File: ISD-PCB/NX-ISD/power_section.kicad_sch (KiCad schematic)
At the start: 31 parts, among them P1 S2B-PH-SM4-TB, Q2 AO3401A, Q3 BC847W, U11 HYCW275-USBC24-050B, U13 RT9193-18GB, U15 USBLC6-2P6, U2 NCP167BMX330TBG, U8 BQ25170DSGR, U9 RT9193-28GB

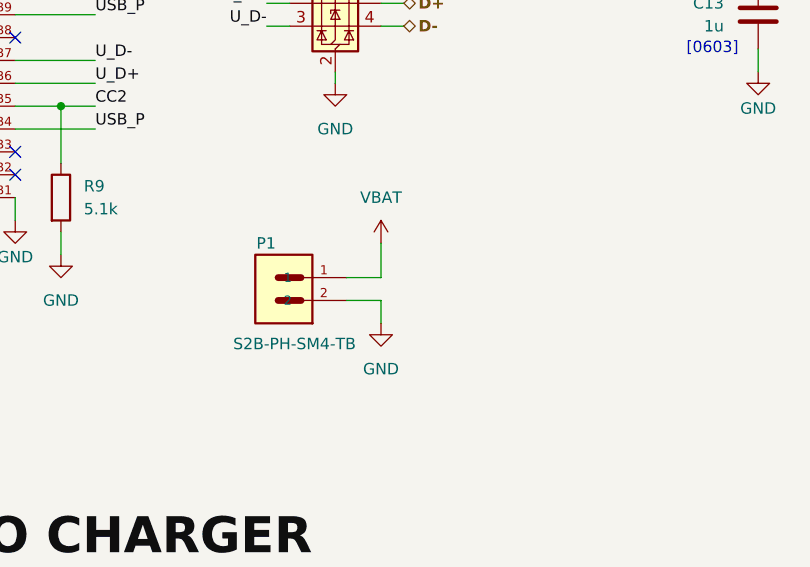
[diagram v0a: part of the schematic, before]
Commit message: v1p1 rework in progress
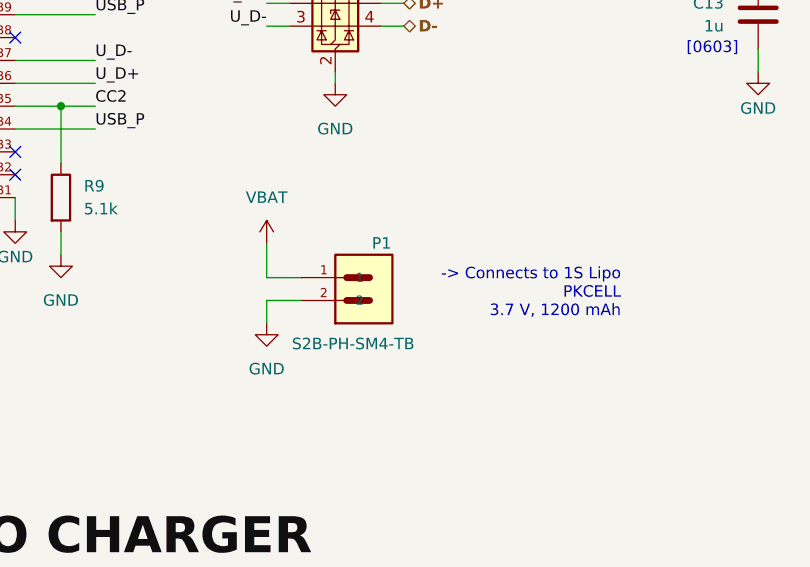
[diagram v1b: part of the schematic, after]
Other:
- note added: "-> Connects to 1S Lipo PKCELL 3.7 V, 1200 mAh"
- moved on the sheet: P1
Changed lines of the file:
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@@
 		)
 	)
+	(text "-> Connects to 1S Lipo\nPKCELL\n3.7 V, 1200 mAh"
+		(exclude_from_sim no)
+		(at 139.7 79.248 0)
+		(effects
+			(font
+				(size 1.27 1.27)
+			)
+			(justify right)
+		)
+	)
 	(text "[0603]"
 		(exclude_from_sim no)
@@
 	(wire
 		(pts
-			(xy 109.22 77.47) (xy 113.03 77.47)
+			(xy 104.14 77.47) (xy 100.33 77.47)
 		)
 		(stroke
@@
 	(wire
 		(pts
-			(xy 109.22 80.01) (xy 113.03 80.01)
+			(xy 104.14 80.01) (xy 100.33 80.01)
 		)
 		(stroke
@@
 	(wire
 		(pts
-			(xy 113.03 73.66) (xy 113.03 77.47)
+			(xy 100.33 73.66) (xy 100.33 77.47)
 		)
 		(stroke
@@
 	(wire
 		(pts
-			(xy 113.03 82.55) (xy 113.03 80.01)
+			(xy 100.33 82.55) (xy 100.33 80.01)
 		)
 		(stroke
@@
 	(symbol
 		(lib_id "power:GND")
-		(at 113.03 82.55 0)
+		(at 100.33 82.55 0)
+		(mirror y)
 		(unit 1)
 		(body_style 1)
@@
 		(fields_autoplaced yes)
 		(property "Reference" "#PWR013"
-			(at 113.03 88.9 0)
+			(at 100.33 88.9 0)
 			(hide yes)
 			(show_name no)
@@
 		)
 		(property "Value" "GND"
-			(at 113.03 87.63 0)
+			(at 100.33 87.63 0)
 			(show_name no)
 			(do_not_autoplace no)
@@
 		)
 		(property "Footprint" ""
-			(at 113.03 82.55 0)
+			(at 100.33 82.55 0)
 			(hide yes)
 			(show_name no)
@@
 		)
 		(property "Datasheet" ""
-			(at 113.03 82.55 0)
+			(at 100.33 82.55 0)
 			(hide yes)
 			(show_name no)
@@
 		)
 		(property "Description" "Power symbol creates a global label with name \"GND\" , ground"
-			(at 113.03 82.55 0)
+			(at 100.33 82.55 0)
 			(hide yes)
 			(show_name no)
@@
 	(symbol
 		(lib_id "S2B-PH-SM4-TB:S2B-PH-SM4-TB")
-		(at 104.14 78.74 0)
-		(mirror y)
+		(at 109.22 78.74 0)
 		(unit 1)
 		(body_style 1)
@@
 		(dnp no)
 		(property "Reference" "P1"
-			(at 101.346 73.66 0)
+			(at 112.014 73.66 0)
 			(show_name no)
 			(do_not_autoplace no)
@@
 		)
 		(property "Value" "S2B-PH-SM4-TB"
-			(at 110.236 84.836 0)
+			(at 103.124 84.836 0)
 			(show_name no)
 			(do_not_autoplace no)
@@
 		)
 		(property "Footprint" "Global Footprints:JST_S2B-PH-SM4-TB"
-			(at 104.14 78.74 0)
+			(at 109.22 78.74 0)
 			(hide yes)
 			(show_name no)
@@
 		)
 		(property "Datasheet" ""
-			(at 104.14 78.74 0)
+			(at 109.22 78.74 0)
 			(hide yes)
 			(show_name no)
@@
 		)
 		(property "Description" ""
-			(at 104.14 78.74 0)
+			(at 109.22 78.74 0)
 			(hide yes)
 			(show_name no)
@@
 		)
 		(property "MF" "JST Sales"
-			(at 104.14 78.74 0)
+			(at 109.22 78.74 0)
 			(hide yes)
 			(show_name no)
@@
 		)
 		(property "Description_1" "Connector Header Surface Mount, Right Angle 2 position 0.079 (2.00mm)"
-			(at 104.14 78.74 0)
+			(at 109.22 78.74 0)
 			(hide yes)
 			(show_name no)
@@
 		)
 		(property "Package" "None"
-			(at 104.14 78.74 0)
+			(at 109.22 78.74 0)
 			(hide yes)
 			(show_name no)
@@
 		)
 		(property "Price" "None"
-			(at 104.14 78.74 0)
+			(at 109.22 78.74 0)
 			(hide yes)
 			(show_name no)
@@
 		)
 		(property "Check_prices" "https://www.snapeda.com/parts/S2B-PH-SM4-TB/JST/view-part/?ref=eda"
-			(at 104.14 78.74 0)
+			(at 109.22 78.74 0)
 			(hide yes)
 			(show_name no)
@@
 		)
 		(property "SnapEDA_Link" "https://www.snapeda.com/parts/S2B-PH-SM4-TB/JST/view-part/?ref=snap"
-			(at 104.14 78.74 0)
+			(at 109.22 78.74 0)
 			(hide yes)
 			(show_name no)
@@
 		)
 		(property "MP" "S2B-PH-SM4-TB"
-			(at 104.14 78.74 0)
+			(at 109.22 78.74 0)
 			(hide yes)
 			(show_name no)
@@
 		)
 		(property "Availability" "In Stock"
-			(at 104.14 78.74 0)
+			(at 109.22 78.74 0)
 			(hide yes)
 			(show_name no)
@@
 		)
 		(property "MANUFACTURER" "JST"
-			(at 104.14 78.74 0)
+			(at 109.22 78.74 0)
 			(hide yes)
 			(show_name no)
@@
 	(symbol
 		(lib_id "power:VBUS")
-		(at 113.03 73.66 0)
+		(at 100.33 73.66 0)
+		(mirror y)
 		(unit 1)
 		(body_style 1)
@@
 		(fields_autoplaced yes)
 		(property "Reference" "#PWR0101"
-			(at 113.03 77.47 0)
+			(at 100.33 77.47 0)
 			(hide yes)
 			(show_name no)
@@
 		)
 		(property "Value" "VBAT"
-			(at 113.03 68.58 0)
+			(at 100.33 68.58 0)
 			(show_name no)
 			(do_not_autoplace no)
@@
 		)
 		(property "Footprint" ""
-			(at 113.03 73.66 0)
+			(at 100.33 73.66 0)
 			(hide yes)
 			(show_name no)
@@
 		)
 		(property "Datasheet" ""
-			(at 113.03 73.66 0)
+			(at 100.33 73.66 0)
 			(hide yes)
 			(show_name no)
@@
 		)
 		(property "Description" "Power symbol creates a global label with name \"VBUS\""
-			(at 113.03 73.66 0)
+			(at 100.33 73.66 0)
 			(hide yes)
 			(show_name no)
